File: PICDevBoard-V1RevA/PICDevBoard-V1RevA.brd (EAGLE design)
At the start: 63 x 42 mm, 18 parts, among them IC1 PIC18F2550, J1 DCJ0202

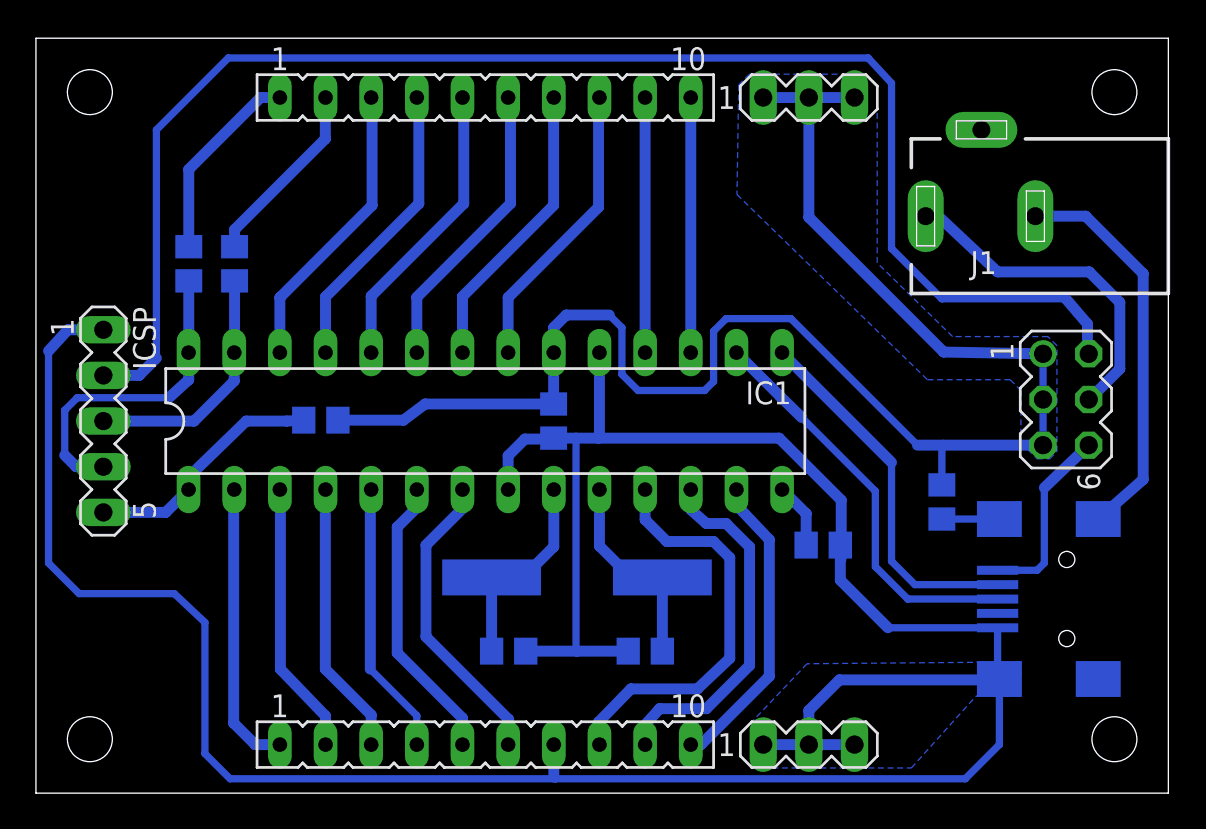
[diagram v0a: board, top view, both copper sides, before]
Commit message: Routing
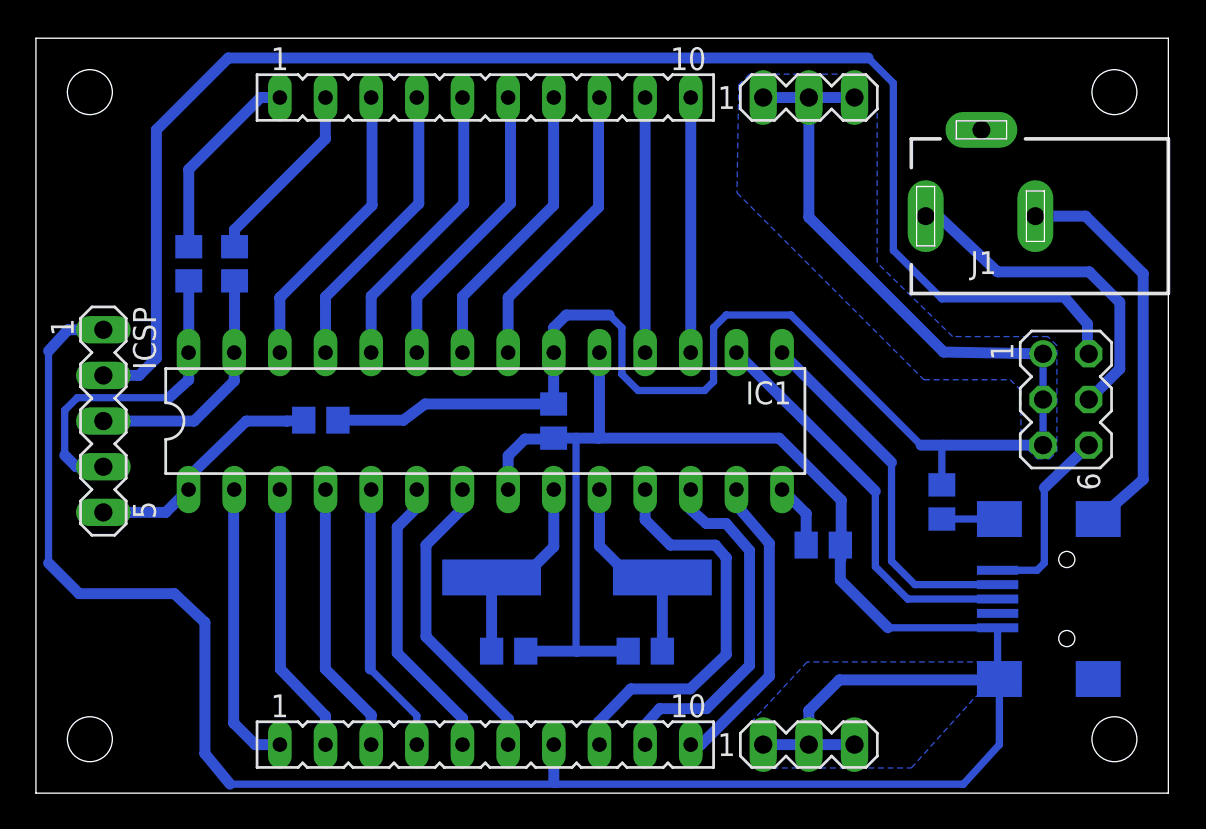
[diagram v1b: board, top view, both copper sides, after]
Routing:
- net GND: track 191.1 -> 191.8 mm
